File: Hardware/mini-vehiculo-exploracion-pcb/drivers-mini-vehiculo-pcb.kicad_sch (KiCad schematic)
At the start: 25 parts, among them J1 Conn_01x08_Pin_drv, J2 Conn_01x02_Pin, J3 Conn_01x03_Pin, J4 Conn_01x02_Motor1, J5 Conn_01x02_Motor2, U1 DRV8873HPWPRQ1, U2 DRV8873HPWPRQ1

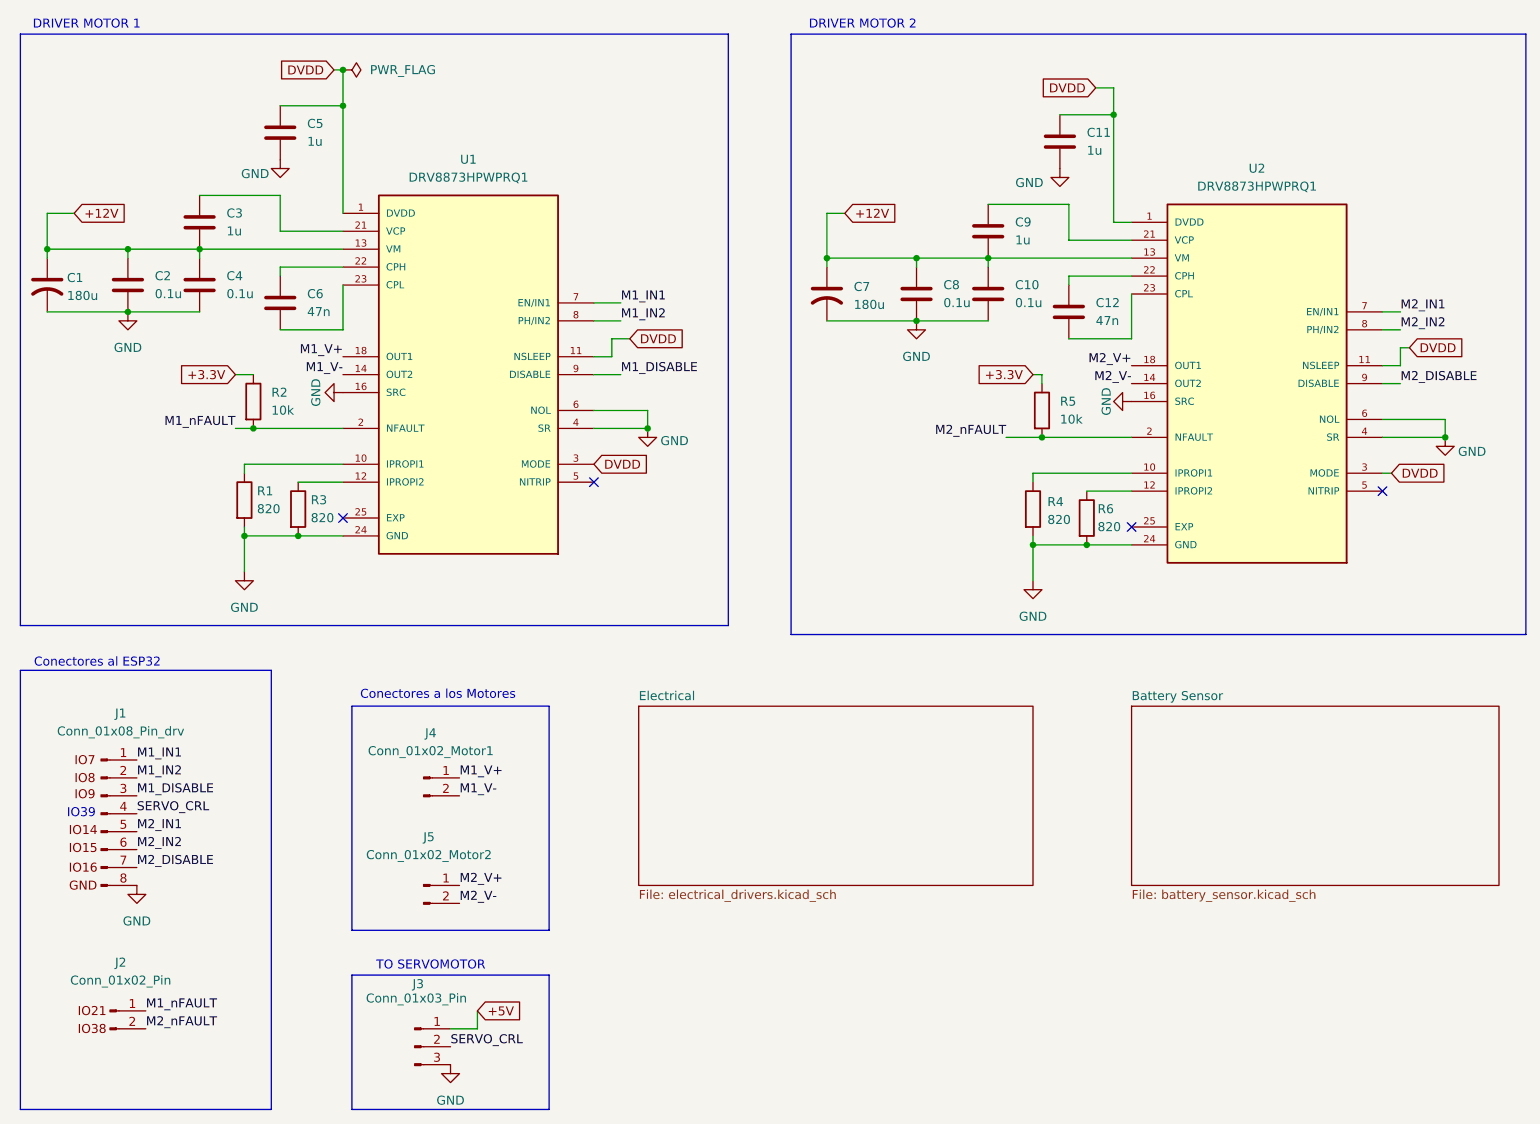
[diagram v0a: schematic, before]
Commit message: changes etc
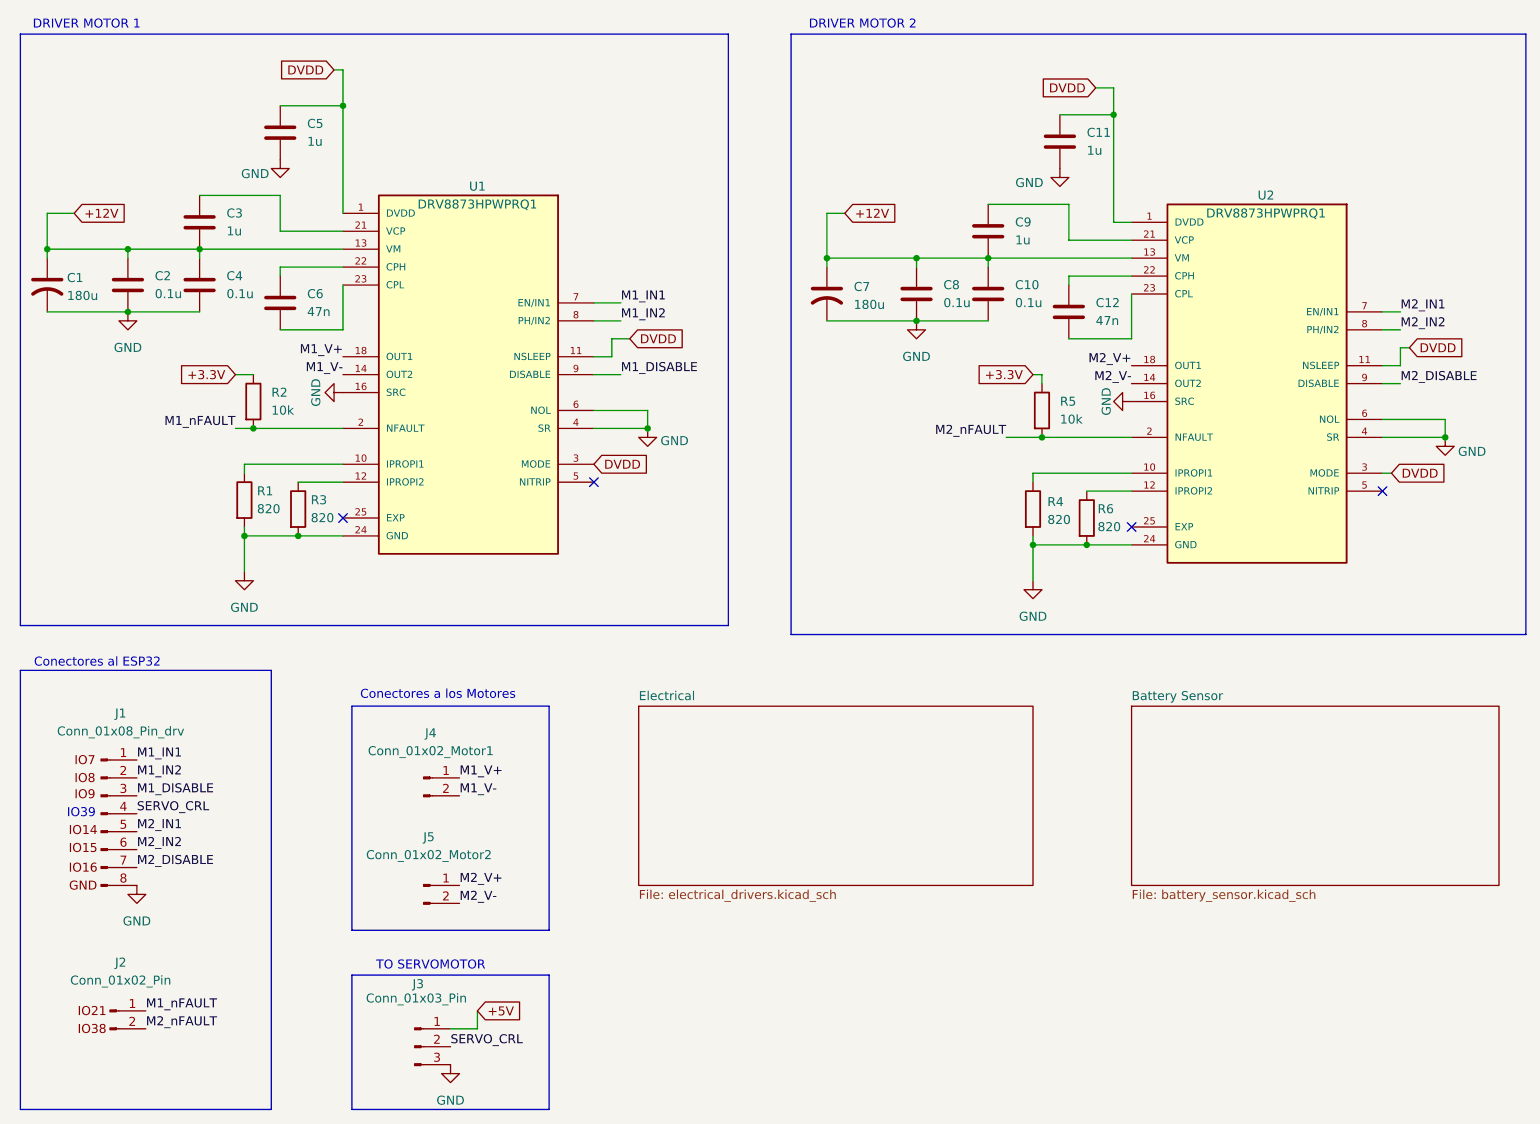
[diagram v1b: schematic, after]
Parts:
- C10, C11, C2, C3, C4, C5, C8, C9: footprint capacitores_driver:CAPC2012X88N -> Capacitor_SMD:C_0805_2012Metric_Pad1.18x1.45mm_HandSolder
- C12, C6: footprint capacitores_driver:CAPC2012X140N -> Capacitor_SMD:C_0805_2012Metric_Pad1.18x1.45mm_HandSolder
- J1: footprint JST_Connectors:JST_8PIN -> Connector_PinSocket_2.54mm:PinSocket_1x08_P2.54mm_Vertical
- J2, J4, J5: footprint (none) -> Connector_PinSocket_2.54mm:PinSocket_1x02_P2.54mm_Vertical
- J3: footprint (none) -> Connector_PinSocket_2.54mm:PinSocket_1x03_P2.54mm_Vertical
- U1, U2: footprint DRV8873HPWPRQ1:DRV8873HPWPRQ1 -> DRV8873HPWPRQ1:SOP65P640X120-25N
